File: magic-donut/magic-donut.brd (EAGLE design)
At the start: 104.1 x 94 mm, 46 parts

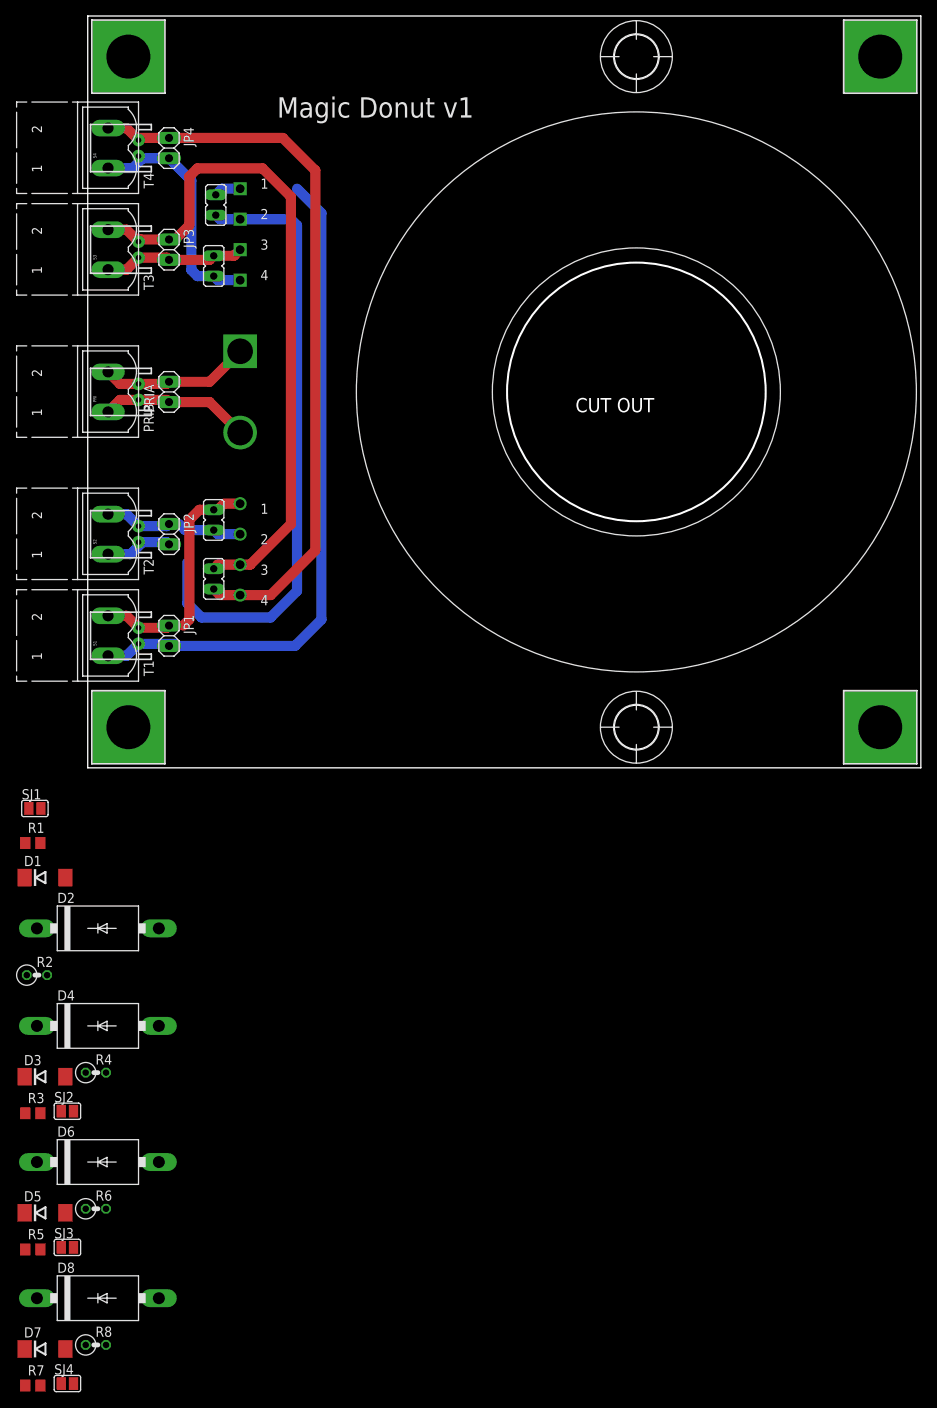
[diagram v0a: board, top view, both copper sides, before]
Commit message: Work with @eranrund
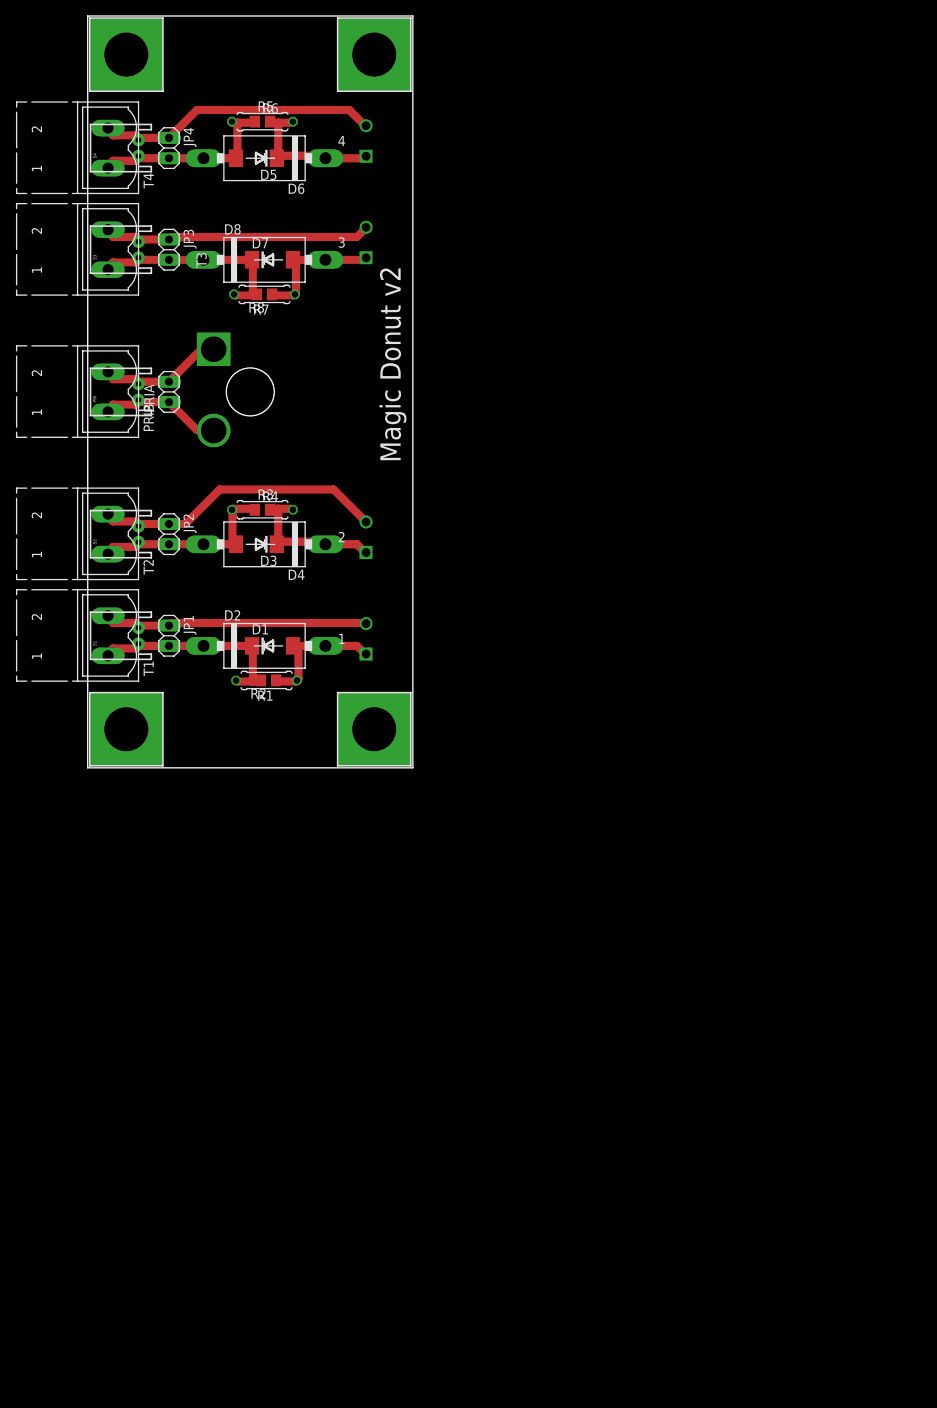
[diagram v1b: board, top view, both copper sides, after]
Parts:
- removed BRIDGE_1_2_A, BRIDGE_1_2_B, BRIDGE_3_4_A, BRIDGE_3_4_B: (no value), jumper:JP1
- removed H1, H2: MOUNT-HOLE5.5, holes:5,5
- removed SJ1, SJ2, SJ3, SJ4: (no value), jumper:SJ
- R2, R4, R6, R8: device rcl:0207/2V -> rcl:0207/7
- moved R5 143.9 mm to (21.8, 80.8)
- moved R7 139.4 mm to (22.1, 59.2), turned to 180 degrees
- moved D7 139.1 mm to (23.1, 63.5)
- moved R6 137.5 mm to (21.8, 80.8)
- moved D5 134.4 mm to (21.1, 76.2), turned to 180 degrees
- moved R8 133.0 mm to (22.1, 59.2), turned to 180 degrees
- moved D8 131.5 mm to (22.1, 63.5)
- moved D6 127.2 mm to (22.1, 76.2), turned to 180 degrees
- moved R3 80.7 mm to (21.8, 32.3)
- moved R4 73.4 mm to (21.8, 32.3)
- moved D3 71.6 mm to (21.1, 27.9), turned to 180 degrees
- moved D4 63.7 mm to (22.1, 27.9), turned to 180 degrees
- moved H7 63.2 mm to (35.8, 4.83)
- moved H8 63.2 mm to (35.8, 89.2)
- moved R2 46.7 mm to (22.4, 10.9), turned to 180 degrees
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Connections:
- removed net N$1: BRIDGE_1_2_A.2, D1.A, D2.A, R1.1, R2.1, SJ1.1, U$1.S1.1
- removed net N$13: D1.C, D2.C, JP1.2, R1.2, R2.2, S1.1, SJ1.2, T1.1
- removed net N$16: D3.C, D4.C, JP2.2, R3.2, R4.2, S2.1, SJ2.2, T2.1
- removed net N$18: D5.C, D6.C, R5.2, R6.2, SJ3.2
- removed net N$19: D7.A, D8.A, R7.1, R8.1, SJ4.1
- removed net N$2: BRIDGE_1_2_B.2, JP1.1, S1.2, T1.2, U$1.S1.2
- removed net N$3: BRIDGE_3_4_A.1, JP4.1, S4.2, T4.2, U$1.S4.2
- removed net N$7: BRIDGE_1_2_B.1, JP2.1, S2.2, T2.2, U$1.S2.2
- new net N$21: JP2.1, S2.2, T2.2, U$1.S2.2
- new net N$22: D3.C, D4.C, R3.2, R4.2, U$1.S2.1
- new net N$23: JP1.1, S1.2, T1.2, U$1.S1.2
- new net N$26: D1.C, D2.C, JP1.2, R1.2, R2.2, S1.1, T1.1
- new net N$9: JP4.1, S4.2, T4.2, U$1.S4.2
- new net S1-1: D1.A, D2.A, R1.1, R2.1, U$1.S1.1
- net N$17: now also JP4.2, S4.1, T4.1; no longer SJ3.1
- net N$20: now also JP3.2, S3.1, T3.1; no longer SJ4.2
- net N$4: now also D5.C, D6.C, R5.2, R6.2; no longer BRIDGE_3_4_B.1, JP4.2, S4.1, T4.1
- net N$5: no longer BRIDGE_3_4_A.2
- net N$6: now also D7.A, D8.A, R7.1, R8.1; no longer BRIDGE_3_4_B.2, JP3.2, S3.1, T3.1
- net N$8: now also JP2.2, S2.1, T2.1; no longer BRIDGE_1_2_A.1, SJ2.1, U$1.S2.1
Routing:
- net N$3: track 91.2 -> 0.00 mm
- net N$13: track 85.4 -> 0.00 mm
- net N$8: track 77.3 -> 24.7 mm
- net N$5: track 85.2 -> 34.1 mm
- net N$21: track 0.00 -> 37.2 mm
- net N$9: track 0.00 -> 35.7 mm
- net N$23: track 0.00 -> 33.6 mm
- net N$2: track 29.1 -> 0.00 mm
- net N$26: track 0.00 -> 26.9 mm
- net N$20: track 0.00 -> 26.9 mm
- net N$17: track 0.00 -> 24.6 mm
- net N$22: track 0.00 -> 19.4 mm
- net S1-1: track 0.00 -> 17.1 mm
- net N$7: track 16.5 -> 0.00 mm
- net N$4: track 30.5 -> 19.2 mm
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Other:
- board size 104.1 x 94 mm -> 40.6 x 94 mm
- board text added: "Magic Donut v2"
- board text removed: "CUT OUT"
- board text removed: "Magic Donut v1"
